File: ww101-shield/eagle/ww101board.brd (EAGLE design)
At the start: 59.1 x 64.6 mm, 57 parts, among them U1 ARDUINO_SHIELDNOHOLESORLABELS

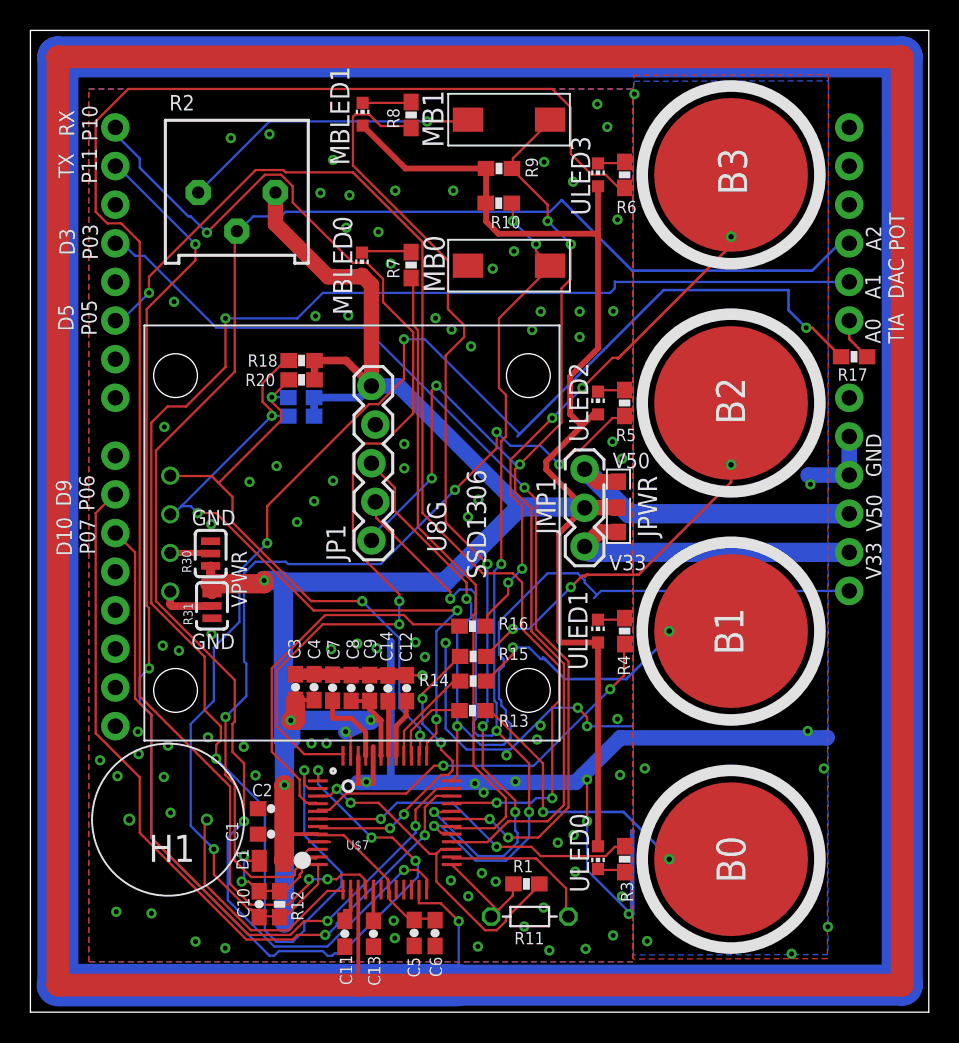
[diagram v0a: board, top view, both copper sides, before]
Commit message: Massive updates to the board
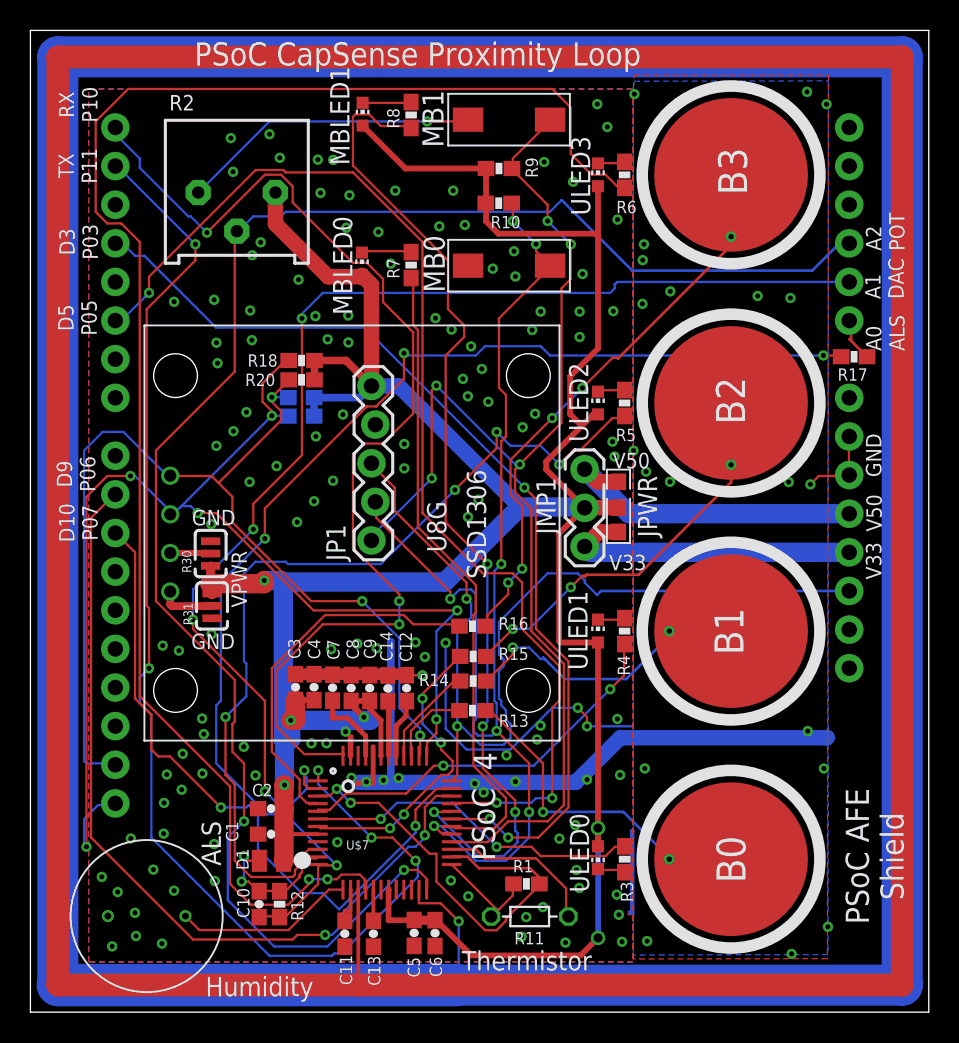
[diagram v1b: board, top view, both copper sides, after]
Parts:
- removed U1: ARDUINO_SHIELDNOHOLESORLABELS, SparkFun-Boards:DUEMILANOVE_SHIELD_NOHOLES_NOLABELS
- added U$1: ARDUINO_R3_SHIELDNOLABELS, SparkFun-Boards:UNO_R3_SHIELD_NOLABELS
- R18, R19, R20, R21: value 10K -> 4.7K
- moved HUMIDITY 6.49 mm to (7.12, 2.76)
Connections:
- removed net THERM-LOW: R11.2, U$7.26
- net A0: now also U$1.A0; no longer U1.A0
- net D10: now also U$1.D10; no longer U1.D10
- net D3: now also U$1.D3; no longer U1.D3
- net D5: now also U$1.D5; no longer U1.D5
- net D9: now also U$1.D9; no longer U1.D9
- net GND: now also R11.2, U$1.GND@0, U$1.GND@1, U$1.GND@2, U$7.27; no longer U1.GND@0, U1.GND@1, U1.GND@2
- net POT: now also U$1.A2; no longer U1.A2
- net SCL: now also U$1.SCL
- net SDA: now also U$1.SDA
- net THERM-REF-HIGH: now also U$7.26; no longer U$7.27
- net UARTRX: now also U$1.TX; no longer U1.TX
- net UARTTX: now also U$1.RX; no longer U1.RX
- net V33: now also U$1.3.3V; no longer U1.3.3V
- net V50: now also U$1.5V; no longer U1.5V
- net VDAC: now also U$1.A1; no longer U1.A1
- net XRES: now also U$1.RES; no longer U1.RES
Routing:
- net SCL: track 46.6 -> 81.4 mm, vias 4 -> 6
- net SDA: track 39.1 -> 69.1 mm
- net VDAC: track 106.3 -> 80.5 mm, vias 3 -> 5
- net THERM-LOW: track 10.4 -> 0.00 mm
- net TIA_OUT: track 90.3 -> 79.9 mm
- net THERM-REF-HIGH: track 22.2 -> 27.8 mm
- net VPWR: track 204.5 -> 209.5 mm, vias 5 -> 7
- net HUMIDITY: track 15.9 -> 11.8 mm
- net D10: track 48.3 -> 45.0 mm
- net D9: track 52.5 -> 55.3 mm
- net GND: track 130.6 -> 129.0 mm, vias 106 -> 151
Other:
- board text added: "4"
- board text added: "A0 ALS"
- board text added: "ALS"
- board text added: "Humidity"
- board text added: "PSoC"
- board text added: "PSoC AFE Shield"
- board text added: "PSoC CapSense Proximity Loop"
- board text added: "PSoC Function P00 MB0 P01 MB1 P02 MBLED0 P03 ARD-D3 P04 MBLED1 P05 ARD-D5 P06 ARD-D9 P07 ARD-D10 P10 ARD-RX P11 ARD-TX"
- board text added: "PSoC Function P12 A0 VDAC P13 THERM-REF-HIGH P14 CapSense B3 P15 CapLED 1 P16 CapLED 0 P17 CapB2 P20 CapLED 2 P21 TIA-IN P22 TIA-Out (A0) P23 Humidity Sensor"
- board text added: "PSoC Function P23 Humidity Sensor P24 Humidity Ref Cap P25 Proximity P26 CapLED 3 P27 SAR Bypass P33 Prox Shield P34 Pot (ARD A3) P35 Therm - MID P36 Therm Ref (1.2V) P37 Therm Low (GND)"
- board text added: "PSoC Function P40 SCL P41 SDA P50 CapSense B0 P51 CapSense B1 P52 CMOD P53 CTANK"
- board text added: "Thermistor"
- board text removed: "A0 TIA"
- board text removed: "H1"
